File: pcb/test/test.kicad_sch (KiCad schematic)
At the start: 17 parts, among them IC1 ADG904BRUZ-REEL7, J1 CONSMA013.062-G, J3 Conn_01x04, U2 TL081

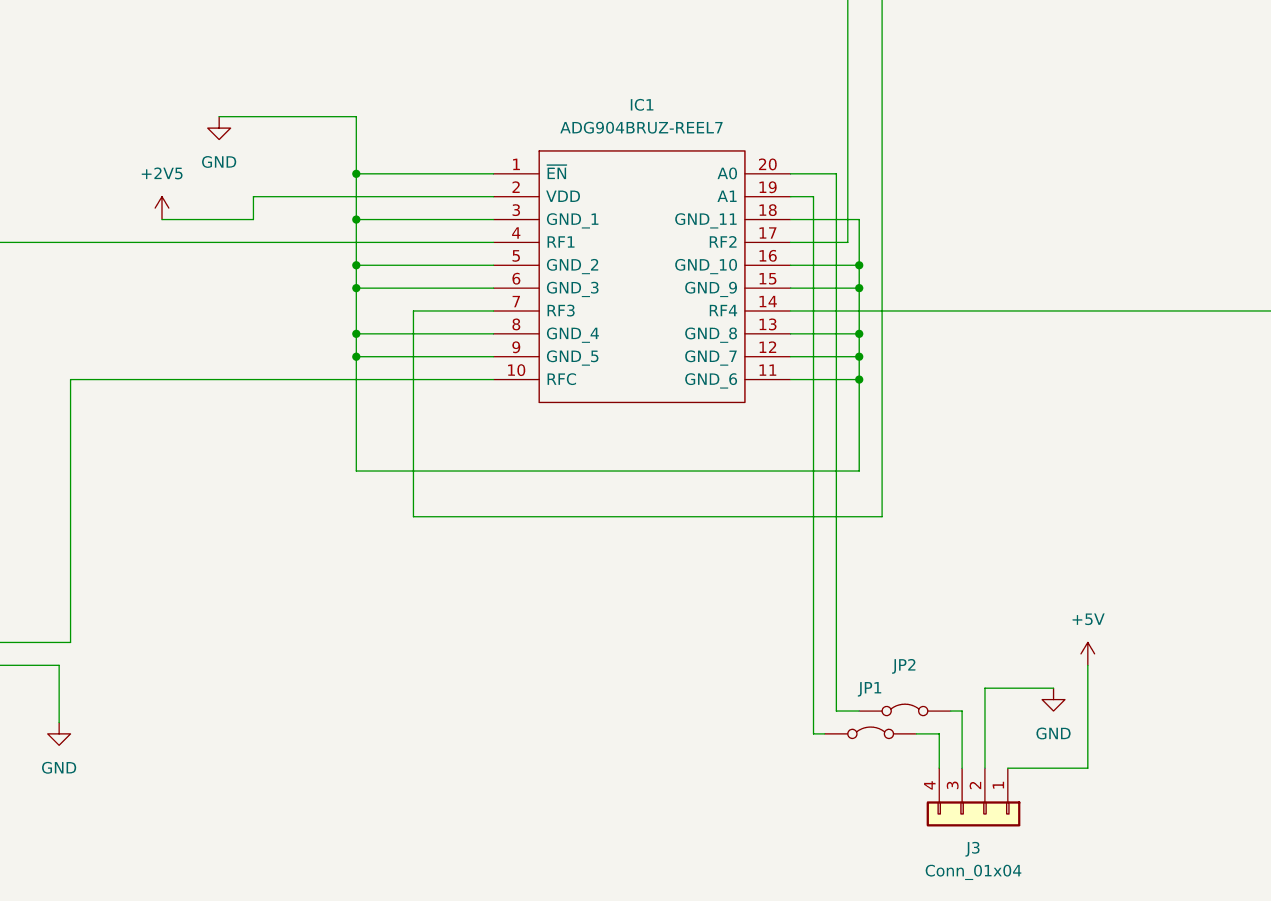
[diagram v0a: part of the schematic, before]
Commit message: beaucoup vias
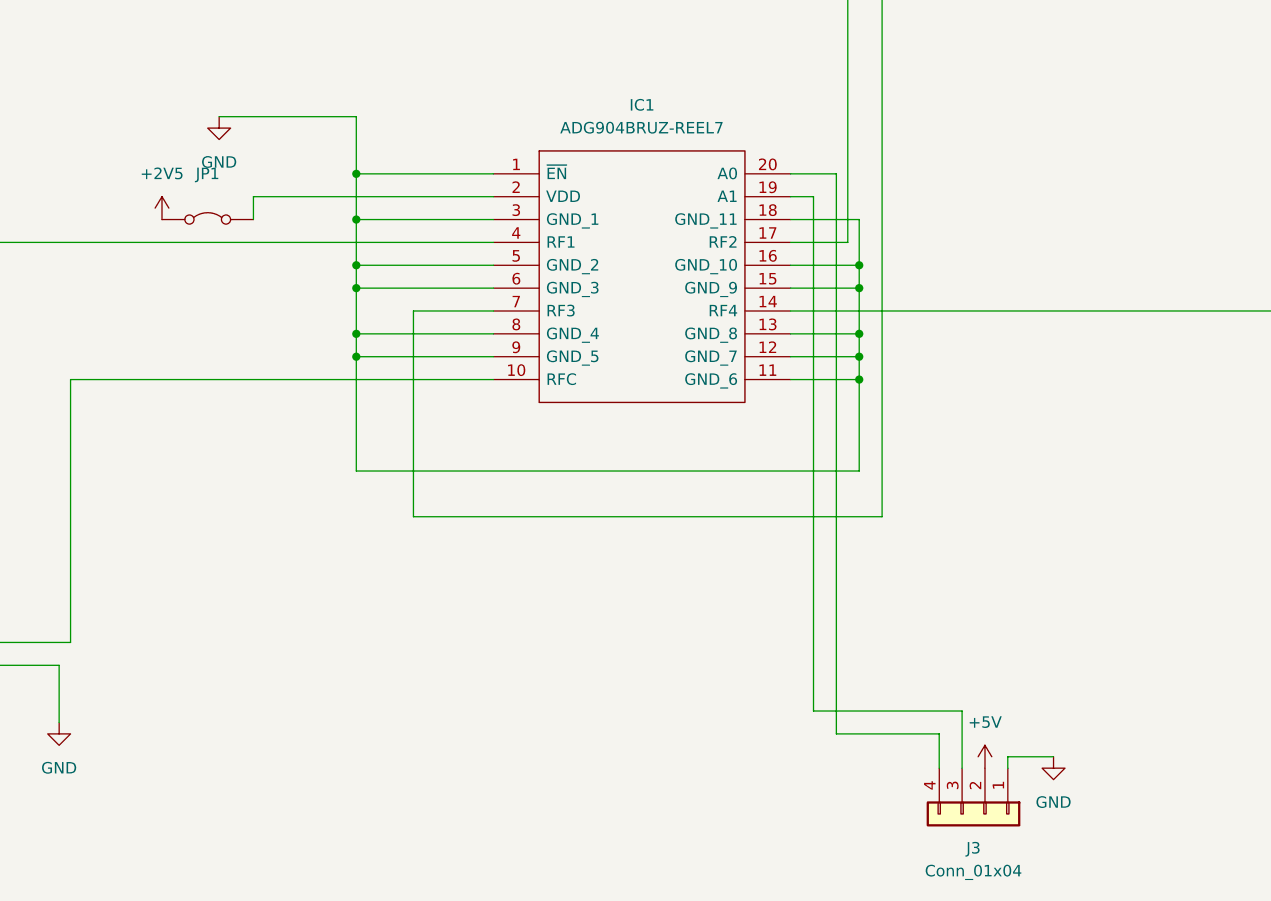
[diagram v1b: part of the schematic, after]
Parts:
- removed JP2: Jumper_2_Bridged, test_footprint_library:jumper20, symbol Jumper:Jumper_2_Bridged
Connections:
- net +2V5: now also JP1.1 (A); no longer IC1.2 (VDD)
- net +5V: now also J3.2 (Pin_2); no longer J3.1 (Pin_1)
- net GND: now also J3.1 (Pin_1); no longer J3.2 (Pin_2)
- net at IC1.20 (A0): now also J3.4 (Pin_4)
- net at J3.3 (Pin_3): now also IC1.19 (A1)
- net at JP1.2 (B): now also IC1.2 (VDD); no longer J3.4 (Pin_4)
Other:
- moved on the sheet: JP1
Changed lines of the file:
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@@
-	(wire
-		(pts
-			(xy 170.18 180.34) (xy 162.56 180.34)
-		)
-		(stroke
-			(width 0)
-			(type default)
-		)
-	)
 	(wire
 		(pts
@@
 	(wire
 		(pts
-			(xy 148.59 182.88) (xy 146.05 182.88)
-		)
-		(stroke
-			(width 0)
-			(type default)
-		)
-	)
-	(wire
-		(pts
 			(xy 172.72 31.75) (xy 179.07 31.75)
 		)
@@
 	(wire
 		(pts
-			(xy 162.56 180.34) (xy 162.56 189.23)
-		)
-		(stroke
-			(width 0)
-			(type default)
-		)
-	)
-	(wire
-		(pts
 			(xy 31.75 27.94) (xy 38.1 27.94)
 		)
@@
 	(wire
 		(pts
-			(xy 160.02 182.88) (xy 158.75 182.88)
-		)
-		(stroke
-			(width 0)
-			(type default)
-		)
-	)
-	(wire
-		(pts
 			(xy 140.97 143.51) (xy 148.59 143.51)
 		)
@@
 	(wire
 		(pts
-			(xy 146.05 182.88) (xy 146.05 123.19)
-		)
-		(stroke
-			(width 0)
-			(type default)
-		)
-	)
-	(wire
-		(pts
 			(xy 92.71 133.35) (xy 92.71 135.89)
 		)
@@
 	(wire
 		(pts
+			(xy 146.05 123.19) (xy 146.05 185.42)
+		)
+		(stroke
+			(width 0)
+			(type default)
+		)
+	)
+	(wire
+		(pts
+			(xy 165.1 189.23) (xy 165.1 187.96)
+		)
+		(stroke
+			(width 0)
+			(type default)
+		)
+	)
+	(wire
+		(pts
+			(xy 143.51 182.88) (xy 160.02 182.88)
+		)
+		(stroke
+			(width 0)
+			(type default)
+		)
+	)
+	(wire
+		(pts
 			(xy 99.06 138.43) (xy 99.06 161.29)
 		)
@@
 	(wire
 		(pts
-			(xy 71.12 128.27) (xy 81.28 128.27)
-		)
-		(stroke
-			(width 0)
-			(type default)
-		)
-	)
-	(wire
-		(pts
 			(xy 148.59 140.97) (xy 148.59 143.51)
 		)
@@
 	(wire
 		(pts
-			(xy 143.51 185.42) (xy 143.51 125.73)
-		)
-		(stroke
-			(width 0)
-			(type default)
-		)
-	)
-	(wire
-		(pts
 			(xy 151.13 161.29) (xy 151.13 31.75)
 		)
@@
 	(wire
 		(pts
-			(xy 157.48 185.42) (xy 154.94 185.42)
-		)
-		(stroke
-			(width 0)
-			(type default)
-		)
-	)
-	(wire
-		(pts
 			(xy 92.71 143.51) (xy 107.95 143.51)
 		)
@@
 	(wire
 		(pts
+			(xy 157.48 185.42) (xy 146.05 185.42)
+		)
+		(stroke
+			(width 0)
+			(type default)
+		)
+	)
+	(wire
+		(pts
 			(xy 148.59 135.89) (xy 148.59 140.97)
 		)
@@
 	(wire
 		(pts
-			(xy 165.1 189.23) (xy 173.99 189.23)
-		)
-		(stroke
-			(width 0)
-			(type default)
-		)
-	)
-	(wire
-		(pts
 			(xy 92.71 140.97) (xy 92.71 143.51)
 		)
@@
 	(wire
 		(pts
+			(xy 165.1 187.96) (xy 170.18 187.96)
+		)
+		(stroke
+			(width 0)
+			(type default)
+		)
+	)
+	(wire
+		(pts
 			(xy 92.71 116.84) (xy 92.71 123.19)
 		)
@@
 	(wire
 		(pts
+			(xy 143.51 182.88) (xy 143.51 125.73)
+		)
+		(stroke
+			(width 0)
+			(type default)
+		)
+	)
+	(wire
+		(pts
 			(xy 99.06 161.29) (xy 151.13 161.29)
 		)
@@
 	(wire
 		(pts
-			(xy 144.78 185.42) (xy 143.51 185.42)
-		)
-		(stroke
-			(width 0)
-			(type default)
-		)
-	)
-	(wire
-		(pts
 			(xy 83.82 48.26) (xy 83.82 30.48)
 		)
@@
 		(pts
 			(xy 208.28 138.43) (xy 208.28 34.29)
-		)
-		(stroke
-			(width 0)
-			(type default)
-		)
-	)
-	(wire
-		(pts
-			(xy 173.99 189.23) (xy 173.99 177.8)
 		)
 		(stroke
@@
 	)
 	(symbol
-		(lib_id "Jumper:Jumper_2_Bridged")
-		(at 153.67 182.88 0)
-		(unit 1)
-		(exclude_from_sim yes)
-		(in_bom yes)
-		(on_board yes)
-		(dnp no)
-		(fields_autoplaced yes)
-		(property "Reference" "JP2"
-			(at 153.67 177.8 0)
-			(effects
-				(font
-					(size 1.27 1.27)
-				)
-			)
-		)
-		(property "Value" "Jumper_2_Bridged"
-			(at 153.67 180.34 0)
-			(effects
-				(font
-					(size 1.27 1.27)
-				)
-				(hide yes)
-			)
-		)
-		(property "Footprint" "test_footprint_library:jumper20"
-			(at 153.67 182.88 0)
-			(effects
-				(font
-					(size 1.27 1.27)
-				)
-				(hide yes)
-			)
-		)
-		(property "Datasheet" "~"
-			(at 153.67 182.88 0)
-			(effects
-				(font
-					(size 1.27 1.27)
-				)
-				(hide yes)
-			)
-		)
-		(property "Description" "Jumper, 2-pole, closed/bridged"
-			(at 153.67 182.88 0)
-			(effects
-				(font
-					(size 1.27 1.27)
-				)
-				(hide yes)
-			)
-		)
-		(pin "2"
-		)
-		(pin "1"
-		)
-		(instances
-			(project "test"
-				(path "/bb1015a8-5dcf-444f-b1dc-3665f721c6b4"
-					(reference "JP2")
-					(unit 1)
-				)
-			)
-		)
-	)
-	(symbol
 		(lib_id "power:GND")
 		(at 241.3 34.29 0)
@@
 	(symbol
 		(lib_id "Jumper:Jumper_2_Bridged")
-		(at 149.86 185.42 0)
+		(at 76.2 128.27 0)
 		(unit 1)
 		(exclude_from_sim yes)
@@
 		(fields_autoplaced yes)
 		(property "Reference" "JP1"
-			(at 149.86 180.34 0)
+			(at 76.2 123.19 0)
 			(effects
 				(font
@@
 		)
 		(property "Value" "Jumper_2_Bridged"
-			(at 149.86 182.88 0)
+			(at 76.2 125.73 0)
 			(effects
 				(font
@@
 		)
 		(property "Footprint" "test_footprint_library:jumper20"
-			(at 149.86 185.42 0)
+			(at 76.2 128.27 0)
 			(effects
 				(font
@@
 		)
 		(property "Datasheet" "~"
-			(at 149.86 185.42 0)
+			(at 76.2 128.27 0)
 			(effects
 				(font
@@
 		)
 		(property "Description" "Jumper, 2-pole, closed/bridged"
-			(at 149.86 185.42 0)
+			(at 76.2 128.27 0)
 			(effects
 				(font
@@
 	(symbol
 		(lib_id "power:+5V")
-		(at 173.99 177.8 0)
+		(at 162.56 189.23 0)
 		(unit 1)
 		(exclude_from_sim no)
@@
 		(fields_autoplaced yes)
 		(property "Reference" "#PWR01"
-			(at 173.99 181.61 0)
+			(at 162.56 193.04 0)
 			(effects
 				(font
@@
 		)
 		(property "Value" "+5V"
-			(at 173.99 172.72 0)
+			(at 162.56 184.15 0)
 			(effects
 				(font
@@
 		)
 		(property "Footprint" ""
-			(at 173.99 177.8 0)
+			(at 162.56 189.23 0)
 			(effects
 				(font
@@
 		)
 		(property "Datasheet" ""
-			(at 173.99 177.8 0)
+			(at 162.56 189.23 0)
 			(effects
 				(font
@@
 		)
 		(property "Description" "Power symbol creates a global label with name \"+5V\""
-			(at 173.99 177.8 0)
+			(at 162.56 189.23 0)
 			(effects
 				(font
@@
 	(symbol
 		(lib_id "power:GND")
-		(at 170.18 180.34 0)
+		(at 170.18 187.96 0)
 		(unit 1)
 		(exclude_from_sim no)
@@
 		(fields_autoplaced yes)
 		(property "Reference" "#PWR08"
-			(at 170.18 186.69 0)
+			(at 170.18 194.31 0)
 			(effects
 				(font
@@
 		)
 		(property "Value" "GND"
-			(at 170.18 185.42 0)
+			(at 170.18 193.04 0)
 			(effects
 				(font
@@
 		)
 		(property "Footprint" ""
-			(at 170.18 180.34 0)
+			(at 170.18 187.96 0)
 			(effects
 				(font
@@
 		)
 		(property "Datasheet" ""
-			(at 170.18 180.34 0)
+			(at 170.18 187.96 0)
 			(effects
 				(font
@@
 		)
 		(property "Description" "Power symbol creates a global label with name \"GND\" , ground"
-			(at 170.18 180.34 0)
-			(effects
-				(font
+			(at 170.18 187.96 0)
+			(effects
+				(font
